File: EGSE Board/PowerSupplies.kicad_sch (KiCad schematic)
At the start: 30 parts, among them U1 VOR2121A8, U2 VOR2121A8, U3 INA238AQDGSRQ1, U4 INA238AQDGSRQ1, U5 INA238AQDGSRQ1, U7 ISO1540, U9 LD1117S33TR_SOT223

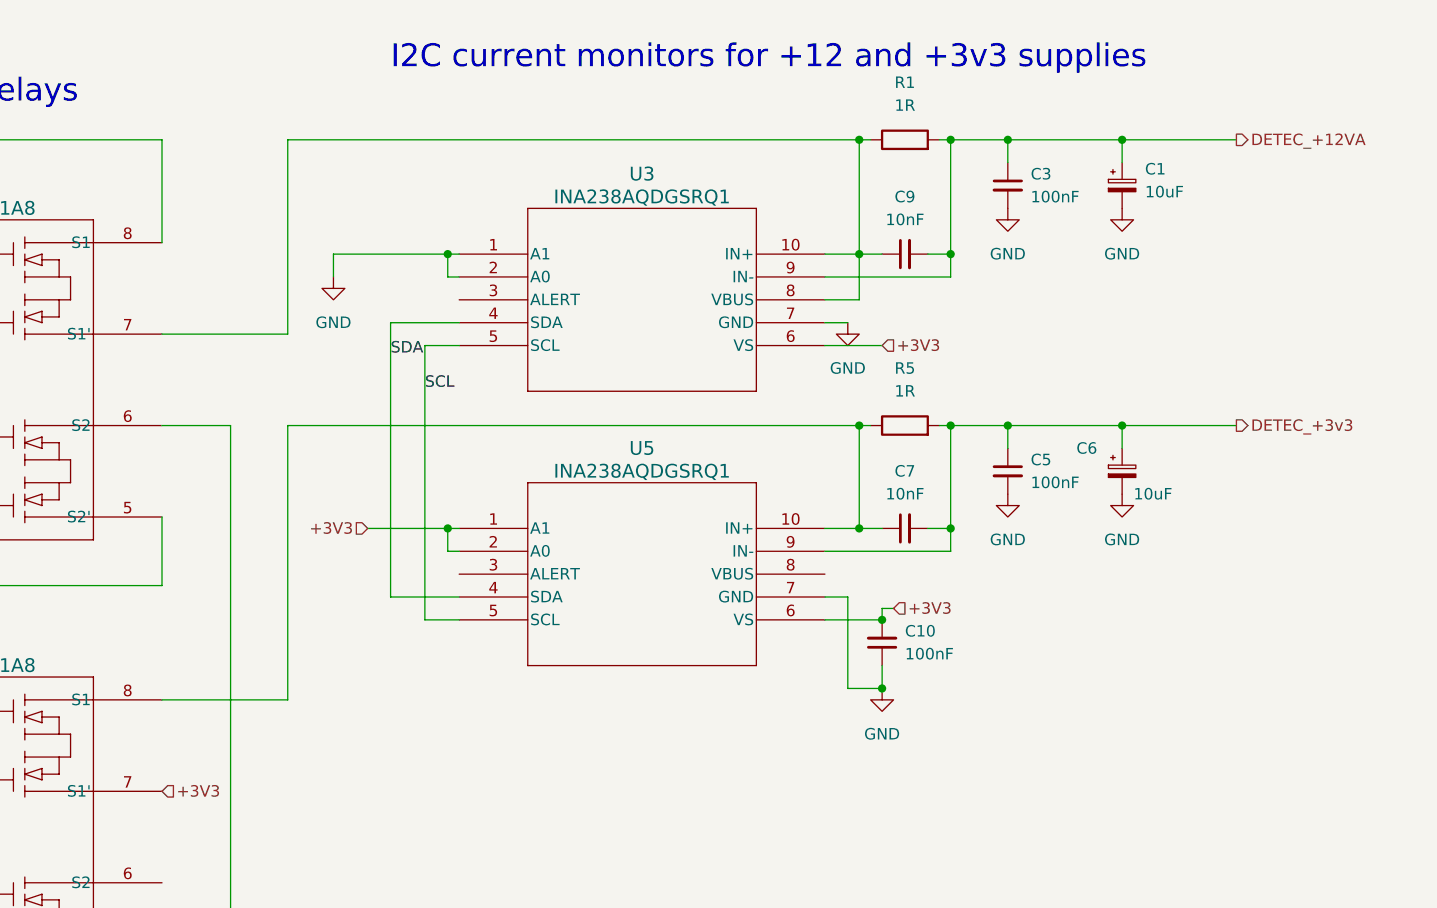
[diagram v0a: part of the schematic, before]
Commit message: Change to heater power
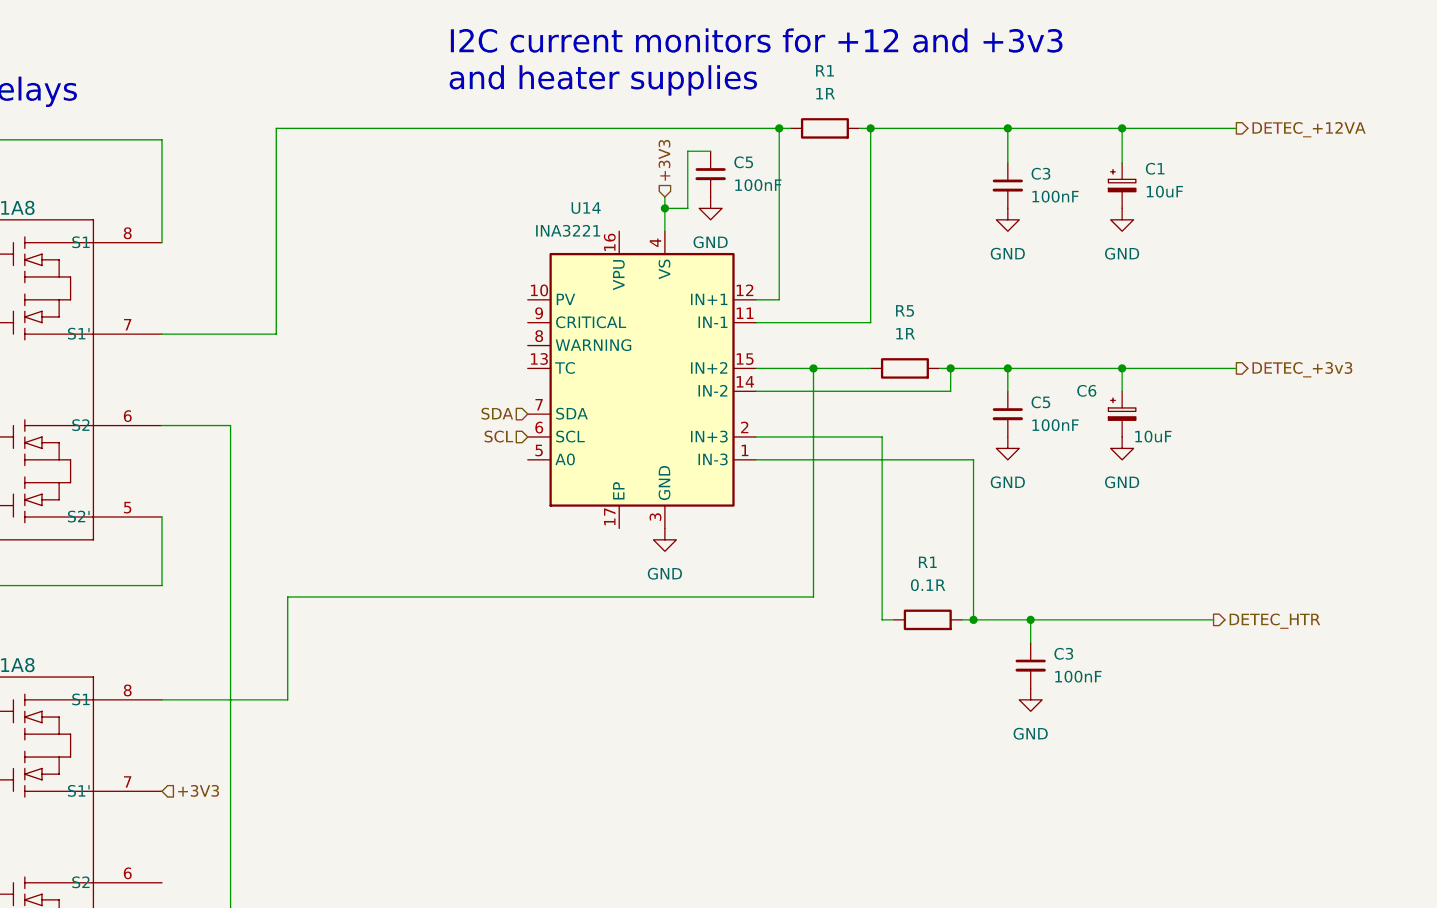
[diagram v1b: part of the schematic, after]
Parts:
- removed C10: 100nF, symbol Device:C_Small
- removed C7, C9: 10nF, symbol Device:C_Small
- removed U3, U5: INA238AQDGSRQ1, Package_SO:VSSOP-10_3x3mm_P0.5mm, symbol Power_Management:INA238AQDGSRQ1
- added C3, C5: 100nF, symbol Device:C_Small
- added R1: 0.1R, symbol Device:R
- added U14: INA3221, Package_DFN_QFN:Texas_RGV_S-PVQFN-N16_EP2.1x2.1mm, symbol Power_Management:INA3221
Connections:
- net +3V3: now also C5.1, U14.4 (VS)
- net DETEC_+12VA: now also U14.11 (IN-1)
- net DETEC_+3v3: now also U14.14 (IN-2)
- net GND: now also C3.2, C5.2, U14.3 (GND)
- net SCL: now also U14.6 (SCL)
- net SDA: now also U14.7 (SDA)
- net at R1.1, U1.7 (S1'): now also U14.12 (IN+1)
- net at R5.1, U2.8 (S1): now also U14.15 (IN+2)
- new net: R1.1, U14.2 (IN+3)
- new net DETEC_HTR: C3.1, R1.2, U14.1 (IN-3)
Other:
- note added: "I2C current monitors for +12 and +3v3 and heater supplies"
- note removed: "I2C current monitors for +12 and +3v3 supplies"
- moved on the sheet: C5, C6, R1, R5
